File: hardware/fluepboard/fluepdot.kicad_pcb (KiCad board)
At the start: 2 copper layers, 65 x 64 mm, 76 parts, among them IC2 IRF7413, IC3 SI4835DDY-T1-E3, J1 Screw_Terminal_01x02, J2 USB_C_Receptacle_USB2.0, J3 Conn_02x17_Odd_Even, J4 Screw_Terminal_01x05, Q1 ULN2803ADWR, Q2 BC847, Q3 BC857, SW1 SW_Push, U1 ESP32-WROOM-32, U2 MCP16301, U3 CP2102N-A01-GQFN24, U4 UMH3N, U5 74HCT595, U6 TBD62783A, U7 74HCT595, U8 TBD62783A, U9 74HCT595

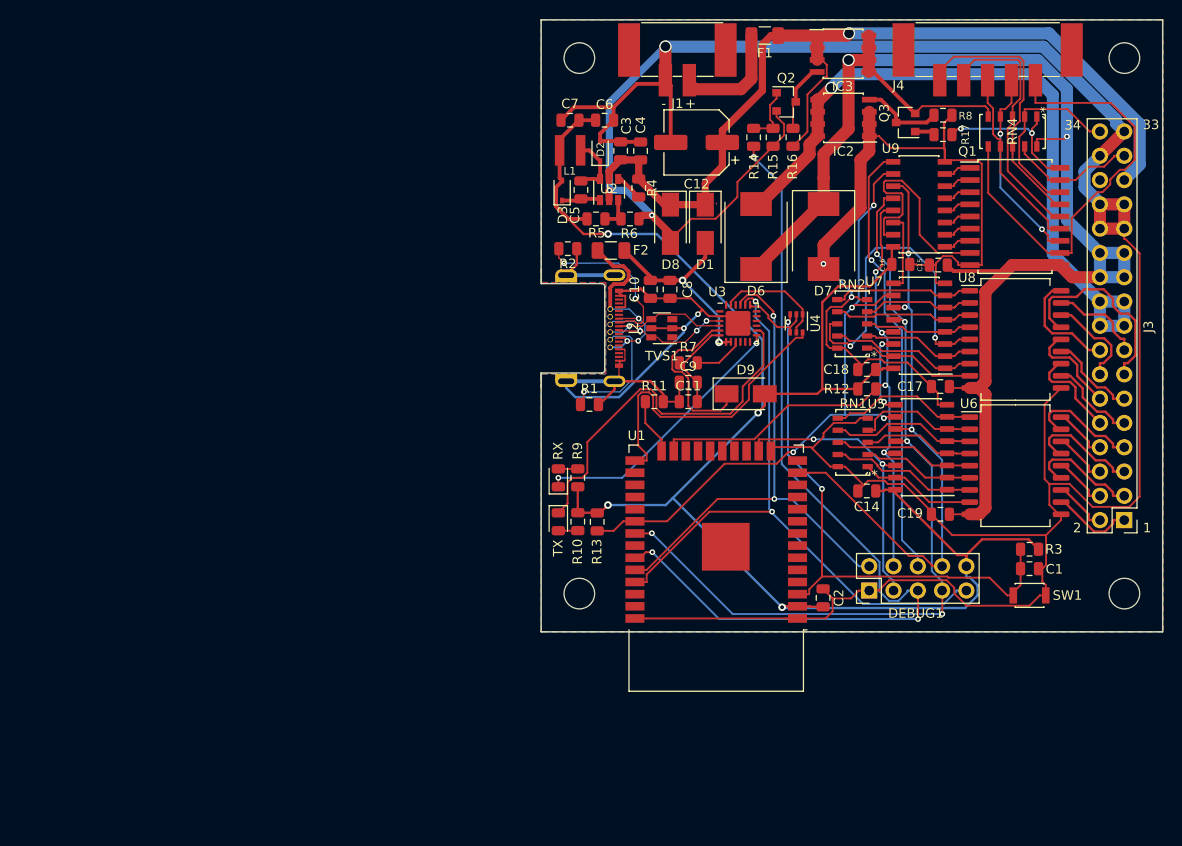
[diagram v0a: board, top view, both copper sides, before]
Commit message: Commit jlcpcb compatible version
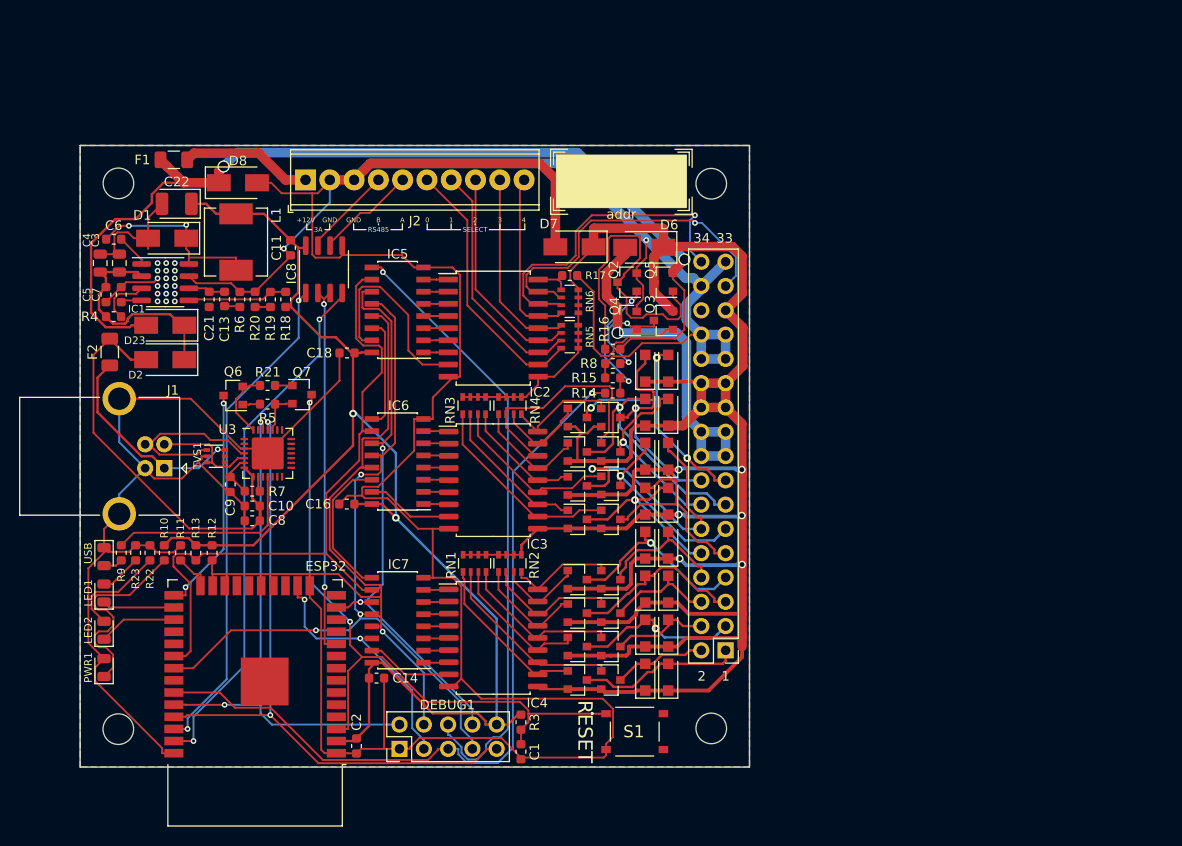
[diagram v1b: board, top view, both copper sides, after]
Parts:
- removed C12: 330uF, Capacitor_SMD:CP_Elec_6.3x7.7
- removed C15, C17, C19: 100nF, Capacitor_SMD:C_0805_2012Metric
- removed J4: Screw_Terminal_01x05, TerminalBlock_Phoenix:TerminalBlock_Phoenix_PTSM-0,5-5-2,5-V-SMD_1x05-1MP_P2.50mm_Vertical
- removed Q1: ULN2803ADWR, Package_SO:SOIC-18W_7.5x11.6mm_P1.27mm
- removed R1, R2: 5k1, Resistor_SMD:R_0805_2012Metric
- removed SW1: SW_Push, B3U-1000P:SW_B3U-1000P
- removed U1: ESP32-WROOM-32, RF_Module:ESP32-WROOM-32
- removed U2: MCP16301, Package_TO_SOT_SMD:SOT-23-6
- removed U4: UMH3N, Package_TO_SOT_SMD:SOT-363_SC-70-6
- removed U5, U7, U9: 74HCT595, Package_SO:SOIC-16_3.9x9.9mm_P1.27mm
- removed U6, U8: TBD62783A, Package_SO:SOP-18_7x12.5mm_P1.27mm
- added C13: 1nF, Capacitor_SMD:C_0603_1608Metric, F.Cu at (45.1, 131.1)
- added C21: 47pF, Capacitor_SMD:C_0603_1608Metric, F.Cu at (43.5, 131.1)
- added C22: 100uF, Capacitor_Tantalum_SMD:CP_EIA-3528-21_Kemet-B, F.Cu at (40.1, 121.1)
- added D10: SM4007PL, Diode_SMD:D_SOD-123F, F.Cu at (91.5, 152.2)
- added D11: SM4007PL, Diode_SMD:D_SOD-123F, F.Cu at (89.1, 166.0)
- added D12: SM4007PL, Diode_SMD:D_SOD-123F, F.Cu at (89.1, 147.5)
- added D13: SM4007PL, Diode_SMD:D_SOD-123F, F.Cu at (91.5, 166.0)
- added D14: SM4007PL, Diode_SMD:D_SOD-123F, F.Cu at (91.5, 147.5)
- added D15: SM4007PL, Diode_SMD:D_SOD-123F, F.Cu at (89.1, 161.4)
- added D16: SM4007PL, Diode_SMD:D_SOD-123F, F.Cu at (89.1, 142.9)
- added D17: SM4007PL, Diode_SMD:D_SOD-123F, F.Cu at (91.5, 161.4)
- added D18: SM4007PL, Diode_SMD:D_SOD-123F, F.Cu at (91.5, 142.9)
- added D19: SM4007PL, Diode_SMD:D_SOD-123F, F.Cu at (89.1, 156.8)
- added D20: SM4007PL, Diode_SMD:D_SOD-123F, F.Cu at (91.5, 138.3)
- added D21: SM4007PL, Diode_SMD:D_SOD-123F, F.Cu at (91.5, 156.8)
- added D22: SM4007PL, Diode_SMD:D_SOD-123F, F.Cu at (89.1, 138.3)
- added D23: SS14, Diode_SMD:D_SMA, F.Cu at (38.9, 133.8)
- added ESP32: ESP32-WROOM-32, RF_Module:ESP32-WROOM-32, F.Cu at (48.3, 170.3)
- added IC1: TPS54331DR, Package_SO:SOIC-8_3.9x4.9mm_P1.27mm, F.Cu at (38.9, 129.3)
- added IC4: ULN2803ADWR, Package_SO:SOIC-18W_7.5x11.6mm_P1.27mm, F.Cu at (73.2, 166.5)
- added IC5: 74HCT595, Package_SO:SOIC-16_3.9x9.9mm_P1.27mm, F.Cu at (63.2, 132.2)
- added IC6: 74HCT595, Package_SO:SOIC-16_3.9x9.9mm_P1.27mm, F.Cu at (63.2, 148.1)
- added IC7: 74HCT595, Package_SO:SOIC-16_3.9x9.9mm_P1.27mm, F.Cu at (63.2, 164.7)
- added IC8: SP3485EN, Package_SO:SOIC-8_3.9x4.9mm_P1.27mm, F.Cu at (55.5, 128.0)
- added LED1: LED1, Diode_SMD:D_0805_2012Metric, F.Cu at (32.5, 161.8)
- added LED2: LED2, Diode_SMD:D_0805_2012Metric, F.Cu at (32.5, 165.7)
- added PWR1: PWR, Diode_SMD:D_0805_2012Metric, F.Cu at (32.5, 169.6)
- added Q10: AO3401A, Package_TO_SOT_SMD:SOT-23, F.Cu at (85.5, 170.9)
- added Q11: AO3401A, Package_TO_SOT_SMD:SOT-23, F.Cu at (82.0, 154.1)
- added Q12: AO3401A, Package_TO_SOT_SMD:SOT-23, F.Cu at (82.0, 167.4)
- added Q13: AO3401A, Package_TO_SOT_SMD:SOT-23, F.Cu at (85.5, 150.6)
- added Q14: AO3401A, Package_TO_SOT_SMD:SOT-23, F.Cu at (85.5, 167.4)
- added Q15: AO3401A, Package_TO_SOT_SMD:SOT-23, F.Cu at (82.0, 150.6)
- added Q16: AO3401A, Package_TO_SOT_SMD:SOT-23, F.Cu at (82.0, 163.9)
- added Q17: AO3401A, Package_TO_SOT_SMD:SOT-23, F.Cu at (82.0, 147.1)
- added Q18: AO3401A, Package_TO_SOT_SMD:SOT-23, F.Cu at (85.5, 163.9)
- added Q19: AO3401A, Package_TO_SOT_SMD:SOT-23, F.Cu at (85.5, 147.1)
- added Q20: AO3401A, Package_TO_SOT_SMD:SOT-23, F.Cu at (82.0, 160.4)
- added Q21: AO3401A, Package_TO_SOT_SMD:SOT-23, F.Cu at (82.0, 143.4)
- added Q22: AO3401A, Package_TO_SOT_SMD:SOT-23, F.Cu at (85.5, 160.4)
- added Q23: AO3401A, Package_TO_SOT_SMD:SOT-23, F.Cu at (85.5, 143.4)
- added Q4: AO3400A, Package_TO_SOT_SMD:SOT-23, F.Cu at (87.2, 133.3)
- added Q5: AO3401A, Package_TO_SOT_SMD:SOT-23, F.Cu at (91.0, 129.3)
- added Q6: SS8050, Package_TO_SOT_SMD:SOT-23, F.Cu at (46.0, 141.2)
- added Q7: SS8050, Package_TO_SOT_SMD:SOT-23, F.Cu at (53.2, 141.1)
- added Q8: AO3401A, Package_TO_SOT_SMD:SOT-23, F.Cu at (82.0, 170.9)
- added Q9: AO3401A, Package_TO_SOT_SMD:SOT-23, F.Cu at (85.5, 154.1)
- added R18: 10k, Resistor_SMD:R_0603_1608Metric, F.Cu at (51.5, 131.1)
- added R19: 3k, Resistor_SMD:R_0603_1608Metric, F.Cu at (49.9, 131.1)
- added R20: 240, Resistor_SMD:R_0603_1608Metric, F.Cu at (48.3, 131.1)
- added R21: 10k, Resistor_SMD:R_0603_1608Metric, F.Cu at (49.6, 140.1)
- added R22: 270, Resistor_SMD:R_0603_1608Metric, F.Cu at (37.3, 157.6)
- added R23: 270, Resistor_SMD:R_0603_1608Metric, F.Cu at (35.8, 157.6)
- added RN3: R_Pack04, Resistor_SMD:R_Array_Convex_4x0603, F.Cu at (71.2, 142.2)
- added RN5: R_Pack04, Resistor_SMD:R_Array_Convex_4x0603, F.Cu at (81.2, 135.0)
- added RN6: R_Pack04, Resistor_SMD:R_Array_Convex_4x0603, F.Cu at (81.2, 131.3)
- added S1: TS-1187A-B-A-B, TS-1187A-B-A-B:TS1187ABAB, F.Cu at (88.0, 176.3)
- C1, C14, C16, C18, C2, C8, C9: footprint Capacitor_SMD:C_0805_2012Metric -> Capacitor_SMD:C_0603_1608Metric
- C10: value 4.7uF -> 1uF; footprint Capacitor_SMD:C_0805_2012Metric -> Capacitor_SMD:C_0603_1608Metric
- C11: value 4.7uF -> 100nF; footprint Capacitor_SMD:C_0805_2012Metric -> Capacitor_SMD:C_0603_1608Metric
- C3, C4: value 10uF -> 4.7uF
- C5: value 100nF -> 10nF; footprint Capacitor_SMD:C_0805_2012Metric -> Capacitor_SMD:C_0603_1608Metric
- C6: value 10uF -> 100nF; footprint Capacitor_SMD:C_0805_2012Metric -> Capacitor_SMD:C_0603_1608Metric
- C7: value 10uF -> 10nF; footprint Capacitor_SMD:C_0805_2012Metric -> Capacitor_SMD:C_0603_1608Metric
- D1, D8: value B140-E3 -> SS34
- D2: value B0540WS-7 -> SS14; footprint Diode_SMD:D_SOD-323 -> Diode_SMD:D_SMA
- D3: value 1N4148 -> SM4007PL; footprint Diode_SMD:D_SOD-323 -> Diode_SMD:D_SOD-123F
- D4: value RX -> USB
- D5: value TX -> SM4007PL; footprint Diode_SMD:D_0805_2012Metric -> Diode_SMD:D_SOD-123F
- D6, D7: footprint Diode_SMD:D_SMC -> Diode_SMD:D_SMA
- D9: value B140-E3 -> SM4007PL; footprint Diode_SMD:D_SMA -> Diode_SMD:D_SOD-123F
- F1: value Fuse -> 3A
- IC2: value IRF7413 -> ULN2803ADWR; footprint Package_SO:SOIC-8_3.9x4.9mm_P1.27mm -> Package_SO:SOIC-18W_7.5x11.6mm_P1.27mm
- IC3: value SI4835DDY-T1-E3 -> ULN2803ADWR; footprint Package_SO:SOIC-8_3.9x4.9mm_P1.27mm -> Package_SO:SOIC-18W_7.5x11.6mm_P1.27mm
- J1: value Screw_Terminal_01x02 -> USB_B; footprint TerminalBlock_Phoenix:TerminalBlock_Phoenix_PTSM-0,5-2-2,5-V-SMD_1x02-1MP_P2.50mm_Vertical -> Connector_USB:USB_B_OST_USB-B1HSxx_Horizontal
- J2: value USB_C_Receptacle_USB2.0 -> Conn_01x10_Female; footprint HIROSE_CX70M-24P1:CX70M-24P1 -> fluepdot:TerminalBlock_Phoenix_MPT-0,5-10-2.54_1x10_P2.54mm_Horizontal
- L1: value 15uH -> 8.2uH; footprint fluepdot:744025150 -> fluepdot:SMD-PIND-6.6x7.1x3.0_1.6x3.0
- Q2: value BC847 -> SS8050
- Q3: value BC857 -> SS8550
- R10: value 270R -> 270; footprint Resistor_SMD:R_0805_2012Metric -> Resistor_SMD:R_0603_1608Metric
- R11, R12, R13, R14, R15, R16, R17, R3, R4, R8, R9: footprint Resistor_SMD:R_0805_2012Metric -> Resistor_SMD:R_0603_1608Metric
- R5: value 31k6 -> 10k; footprint Resistor_SMD:R_0805_2012Metric -> Resistor_SMD:R_0603_1608Metric
- R6: value 10k -> 30k; footprint Resistor_SMD:R_0805_2012Metric -> Resistor_SMD:R_0603_1608Metric
- R7: value 1k -> 4.7k; footprint Resistor_SMD:R_0805_2012Metric -> Resistor_SMD:R_0603_1608Metric
- RN1, RN2, RN4: value EXB-A10P103J -> R_Pack04; footprint EXB-A10P103J:EXB-A10P103J -> Resistor_SMD:R_Array_Convex_4x0603
- TVS1: value SN65220DBVR -> SMF05CT1G; footprint Package_TO_SOT_SMD:SOT-23-6 -> Package_TO_SOT_SMD:SOT-363_SC-70-6
- U3: value CP2102N-A01-GQFN24 -> CP2102N-A01-GQFN28; footprint Package_DFN_QFN:QFN-24-1EP_4x4mm_P0.5mm_EP2.6x2.6mm -> Package_DFN_QFN:QFN-28-1EP_5x5mm_P0.5mm_EP3.35x3.35mm
- moved R12 70.6 mm to (43.8, 157.6), turned to 270 degrees
- moved J1 68.6 mm to (38.8, 148.8), turned to 180 degrees
- moved F1 63.2 mm to (39.8, 116.5), turned to 0 degrees
- moved C16 63.1 mm to (57.9, 152.5), turned to 180 degrees
- moved RN4 59.9 mm to (75.0, 142.2), turned to 90 degrees
- moved C4 57.7 mm to (32.1, 127.3)
- moved IC3 57.7 mm to (73.2, 150.0)
- moved R4 56.5 mm to (33.5, 132.9), turned to 0 degrees
- moved C1 56.5 mm to (76.1, 178.4), turned to 270 degrees
- moved D1 56.3 mm to (39.1, 124.7), turned to 180 degrees
- moved R3 56.2 mm to (76.1, 175.3), turned to 270 degrees
- moved C14 54.9 mm to (61.0, 170.7), turned to 0 degrees
- moved C18 54.4 mm to (57.9, 136.7)
- moved C3 53.7 mm to (34.1, 127.3)
- moved F2 53.5 mm to (33.1, 136.6), turned to 270 degrees
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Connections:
- C11 pad 1: GND -> +3V3
- C11 pad 2: Net-(C11-Pad2) -> GND
- C3 pad 1: +12V -> Net-(C3-Pad1)
- C4 pad 1: +12V -> Net-(C3-Pad1)
- C5 pad 1: Net-(C5-Pad1) -> Net-(C3-Pad1)
- C5 pad 2: Net-(C5-Pad2) -> GND
- C6 pad 1: +3V3 -> Net-(C6-Pad1)
- C6 pad 2: GND -> Net-(C6-Pad2)
- C7 pad 1: +3V3 -> Net-(C7-Pad1)
- C9 pad 2: Net-(C11-Pad2) -> Net-(C9-Pad2)
- D1 pad 1: +12V -> Net-(C6-Pad1)
- D1 pad 2: VUSB -> GND
- D2 pad 1: Net-(C5-Pad2) -> Net-(C3-Pad1)
- D2 pad 2: GND -> VUSB
- D3 pad 1: Net-(C5-Pad1) -> VFlipdot
- D3 pad 2: +3V3 -> Y0_OUT
- D4 pad 1: Net-(D4-Pad1) -> GND
- D5 pad 1: Net-(D5-Pad1) -> VFlipdot
- D5 pad 2: Net-(D5-Pad2) -> Y8_OUT
- D9 pad 1: Net-(D9-Pad1) -> VFlipdot
- D9 pad 2: +3V3 -> Y1_OUT
- F1 pad 2: /Powersupply/V_in -> V_in
- IC2 pad 1: GND -> CLEAR_INT
- IC2 pad 2: GND -> RESET_INT
- IC2 pad 3: GND -> CLOCK_INT
- IC2 pad 4: Net-(IC2-Pad4) -> SELECT4_INT
- IC2 pad 5: CLEAR_OUT -> SELECT3_INT
- IC2 pad 6: CLEAR_OUT -> SELECT2_INT
- IC2 pad 7: CLEAR_OUT -> SELECT1_INT
- IC2 pad 8: CLEAR_OUT -> SELECT0_INT
- IC3 pad 1: +12V -> Y15_INT
- IC3 pad 2: +12V -> Y14_INT
- IC3 pad 3: +12V -> Y13_INT
- IC3 pad 4: Net-(IC3-Pad4) -> Y12_INT
- IC3 pad 5: VFlipdot -> Y11_INT
- IC3 pad 6: VFlipdot -> Y10_INT
- IC3 pad 7: VFlipdot -> Y9_INT
- IC3 pad 8: VFlipdot -> Y8_INT
- J1 pad 1: GND -> /USB2Serial/VBus
- J1 pad 2: /Powersupply/V_in -> /USB2Serial/D-
- J3 pad 29: +12V -> VFlipdot
- J3 pad 30: Net-(J3-Pad30) -> (no net)
- L1 pad 1: Net-(C5-Pad2) -> Net-(C6-Pad1)
- Q2 pad 3: Net-(IC3-Pad4) -> Net-(Q2-Pad3)
- Q3 pad 3: Net-(IC2-Pad4) -> Net-(Q3-Pad3)
- R10 pad 2: Net-(D5-Pad2) -> Net-(PWR1-Pad1)
- R16 pad 2: Net-(IC3-Pad4) -> Net-(Q2-Pad3)
- R4 pad 1: +12V -> Net-(C3-Pad1)
- R5 pad 1: +3V3 -> Net-(Q6-Pad1)
- R5 pad 2: Vfb -> /Reset circuitry/RTS
- R6 pad 1: Vfb -> Net-(C13-Pad2)
- R7 pad 1: Net-(C11-Pad2) -> Net-(C9-Pad2)
- R8 pad 1: Net-(IC2-Pad4) -> Net-(Q3-Pad3)
- R9 pad 1: +3V3 -> Net-(D4-Pad2)
- R9 pad 2: Net-(D4-Pad2) -> Net-(R9-Pad2)
- RN1 pad 2: Y2 -> Y1
- RN1 pad 3: Y4 -> Y2
- RN1 pad 4: Y6 -> Y3
- RN1 pad 5: GND -> VFlipdot
- RN1 pad 6: Y7 -> VFlipdot
- RN1 pad 7: Y5 -> VFlipdot
- RN1 pad 8: Y3 -> VFlipdot
- RN2 pad 1: Y8 -> Y4
- RN2 pad 2: Y10 -> Y5
- RN2 pad 3: Y12 -> Y6
- RN2 pad 4: Y14 -> Y7
- RN2 pad 5: GND -> VFlipdot
- RN2 pad 6: Y15 -> VFlipdot
- RN2 pad 7: Y13 -> VFlipdot
- RN2 pad 8: Y11 -> VFlipdot
- RN4 pad 1: CLEAR_GATE -> Y12
- RN4 pad 2: CLOCK_OUT -> Y13
- RN4 pad 3: /Flipdot Control Unit/SELECT3_OUT -> Y14
- RN4 pad 4: /Flipdot Control Unit/SELECT1_OUT -> Y15
- RN4 pad 6: /Flipdot Control Unit/SELECT0_OUT -> VFlipdot
- RN4 pad 7: /Flipdot Control Unit/SELECT2_OUT -> VFlipdot
- RN4 pad 8: /Flipdot Control Unit/SELECT4_OUT -> VFlipdot
- TVS1 pad 1: Net-(TVS1-Pad1) -> /USB2Serial/D+
- TVS1 pad 3: Net-(TVS1-Pad3) -> /USB2Serial/D-
- TVS1 pad 4: /USB2Serial/D+ -> (no net)
- TVS1 pad 5: GND -> (no net)
- TVS1 pad 6: /USB2Serial/D- -> /USB2Serial/VBus
- U3 pad 1: Net-(U3-Pad1) -> (no net)
- U3 pad 10: Net-(U3-Pad10) -> (no net)
- U3 pad 11: Net-(U3-Pad11) -> Net-(R9-Pad2)
- U3 pad 12: Net-(U3-Pad12) -> (no net)
- U3 pad 13: Net-(D4-Pad1) -> (no net)
- U3 pad 14: Net-(D5-Pad1) -> (no net)
- U3 pad 15: Net-(U3-Pad15) -> (no net)
- U3 pad 16: Net-(U3-Pad16) -> (no net)
- U3 pad 17: Net-(U3-Pad17) -> (no net)
- U3 pad 18: Net-(U3-Pad18) -> (no net)
- U3 pad 19: /Reset circuitry/RTS -> (no net)
- U3 pad 2: GND -> (no net)
- U3 pad 20: TXD0 -> (no net)
- U3 pad 21: RXD0 -> (no net)
- U3 pad 22: Net-(U3-Pad22) -> (no net)
- U3 pad 23: /Reset circuitry/DTR -> (no net)
- U3 pad 24: Net-(U3-Pad24) -> /Reset circuitry/RTS
- U3 pad 25: GND -> TXD0
- U3 pad 3: /USB2Serial/D- -> GND
- U3 pad 5: Net-(D9-Pad1) -> /USB2Serial/D-
- U3 pad 6: Net-(C11-Pad2) -> Net-(C9-Pad2)
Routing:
- net VFlipdot: track 155.7 -> 274.0 mm, vias 2 -> 6
- net RS485_TXD: track 0.00 -> 55.4 mm, vias 0 -> 2
- net RS485_RXD: track 0.00 -> 52.1 mm, vias 0 -> 2
- net /Flipdot Control Unit/SELECT0_OUT: track 46.0 -> 0.00 mm
- net +3V3: track 179.5 -> 139.6 mm, vias 4 -> 2
- net RS485_RTS: track 0.00 -> 39.1 mm, vias 0 -> 2
- net Net-(D5-Pad1): track 39.1 -> 0.00 mm
- net CLEAR_OUT: track 74.3 -> 38.3 mm
- net Net-(Q2-Pad3): track 0.00 -> 34.4 mm
- net GND: track 468.9 -> 437.8 mm, vias 7 -> 20
- net Net-(D4-Pad1): track 28.3 -> 0.00 mm, vias 2 -> 0
- net /Flipdot Control Unit/SELECT4_OUT: track 28.3 -> 0.00 mm
- net SELECT0_OUT: track 0.00 -> 28.0 mm
- net /Flipdot Control Unit/SELECT3_OUT: track 26.9 -> 0.00 mm
- net SELECT1_OUT: track 0.00 -> 25.4 mm
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- added copper zone on B.Cu, net +3V3
- added copper zone on F.Cu, net GND
- removed copper zone on F.Cu, net +3V3
- removed copper zone on B.Cu, net GND
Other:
- board size 65 x 64 mm -> 70 x 65 mm
- board text added: "+12V"
- board text added: "0"
- board text added: "3"
- board text added: "3A"
- board text added: "4"
- board text added: "A"
- board text added: "B"
- board text added: "GND"
- board text added: "RESET"
- board text added: "RS485"
- board text added: "SELECT"
- board text added: "addr"
- board text removed: "+"
- board text removed: "-"
